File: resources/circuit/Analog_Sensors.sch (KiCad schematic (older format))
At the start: 43 parts, among them J3 Screw_Terminal_1x08, Q10 BSS138, Q11 BSS138, Q7 BSS138, Q8 BSS138, Q9 BSS138, U13 Airspeed, U14 Static Pressure, U15 MAP Pressure, U8 MCP3008, U9 MCP3008

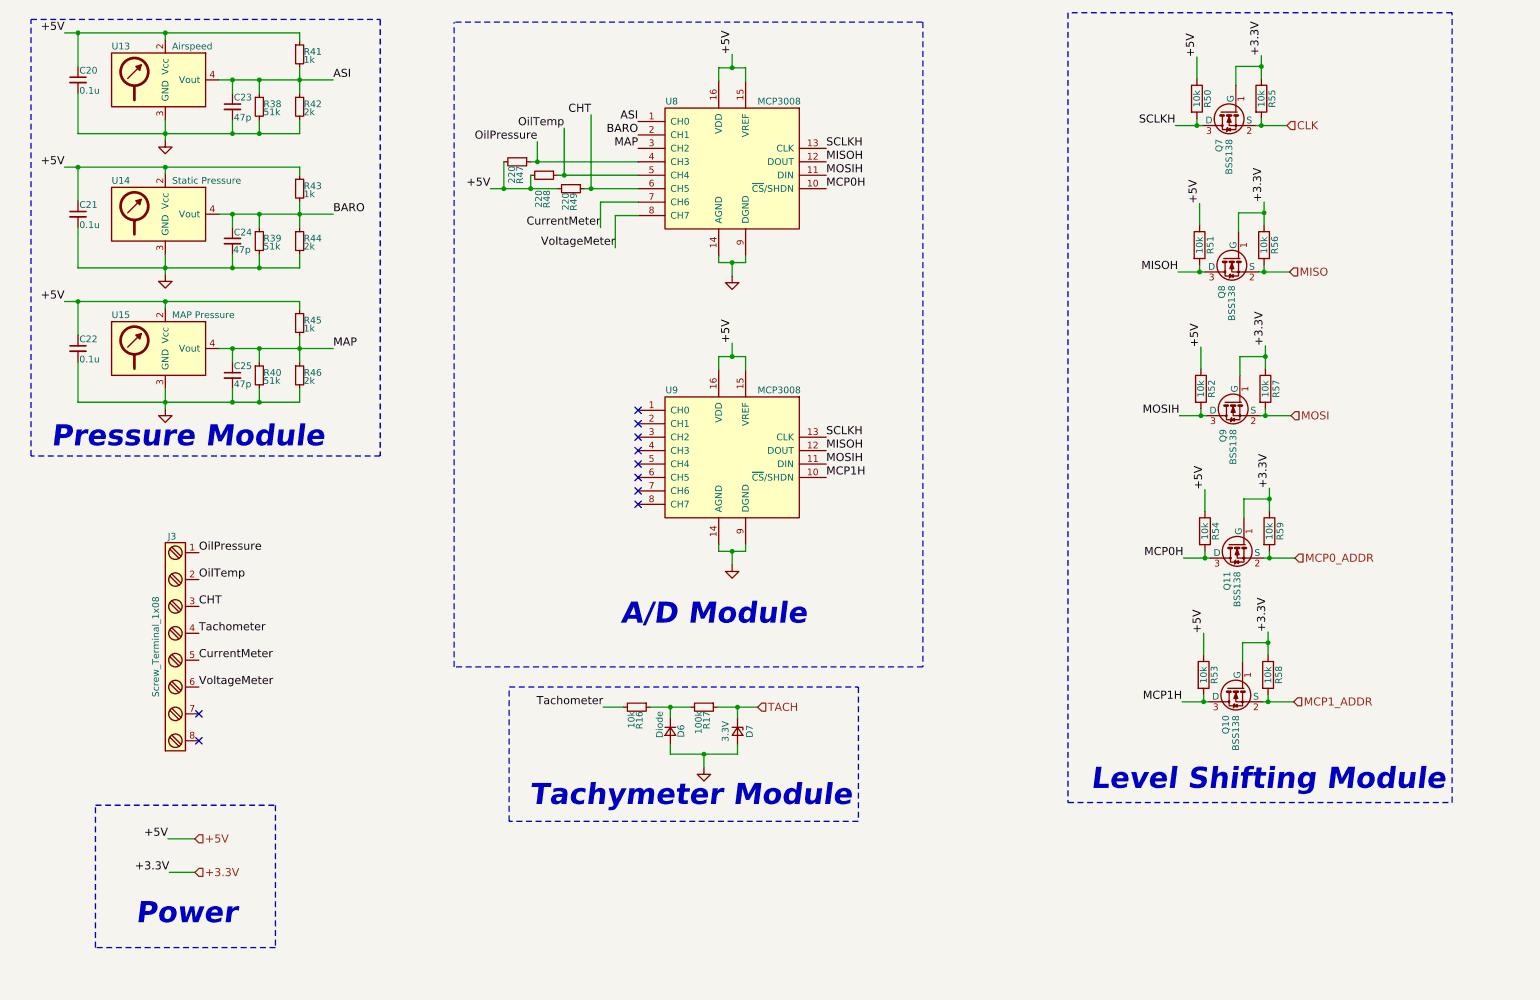
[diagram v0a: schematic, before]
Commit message: Another RPM reading solution
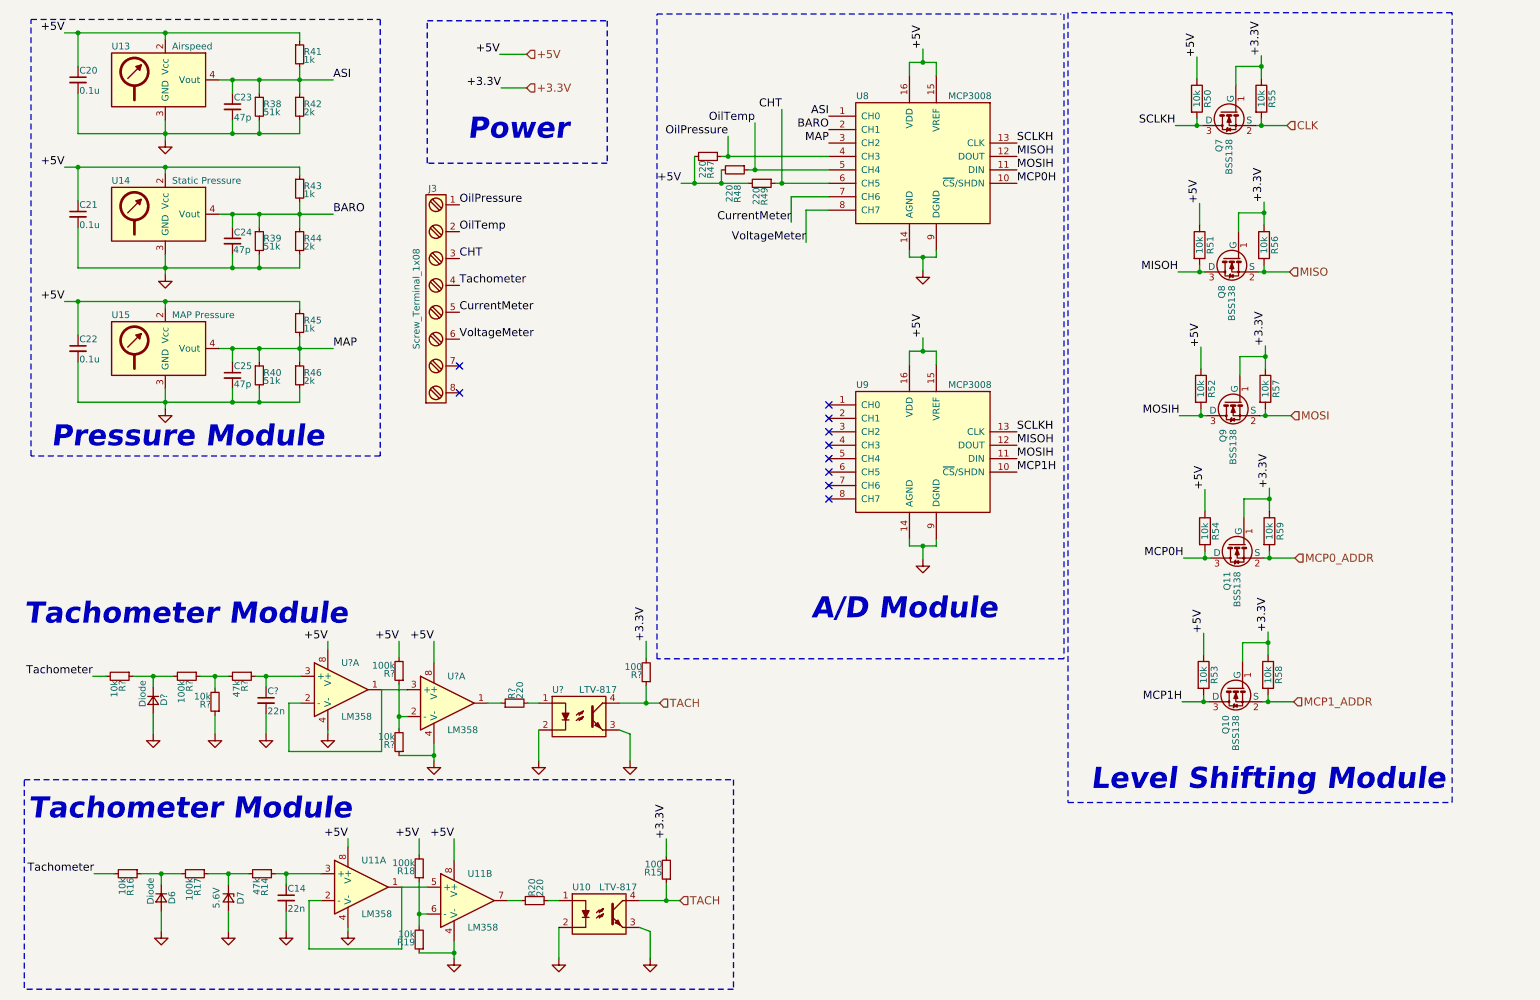
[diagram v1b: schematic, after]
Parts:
- added C14, C?: 22n, symbol C_Small
- added D?: Diode, Diodes_SMD:D_0603, symbol D_Small
- added R14, R?: 47k, symbol R_Small
- added R15, R?: 100, symbol R_Small
- added R18, R? (x2): 100k, Resistors_SMD:R_0603, symbol R_Small
- added R19, R? (x3): 10k, Resistors_SMD:R_0603, symbol R_Small
- added R20, R?: 220, Resistors_SMD:R_0603, symbol R_Small
- added U10, U?: LTV-817, Housings_DIP:DIP-4_W7.62mm, symbol LTV-817
- added U11, U? (x2): LM358, symbol LM358
- D7: value 3.3V -> 5.6V
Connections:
- net +3.3V: now also R15.2, R?.2
- net +5V: now also R18.2, R?.2, U11.8 (V+), U11.8 (V+), U?.8 (V+), U?.8 (V+)
- net GND: now also C14.2, C?.2, D?.2 (A), R19.1, R?.1, R?.1, U10.2, U10.3, U11.4 (V-), U11.4 (V-), U?.2, U?.3, U?.4 (V-), U?.4 (V-)
- net TACH: now also R15.1, R?.1, U10.4, U?.4; no longer D7.1 (K), R17.1
- net Tachometer: now also R?.2
- new net: D7.1 (K), R14.2, R17.1
- new net: C14.1, R14.1, U11.3 (+)
- new net: R20.2, U10.1
- new net: U11.1, U11.2 (-), U11.5 (+)
- new net: R18.1, R19.2, U11.6 (-)
- new net: R20.1, U11.7
- new net: R?.2, U?.1
- new net: U?.1, U?.2 (-), U?.3 (+)
- new net: C?.1, R?.1, U?.3 (+)
- new net: R?.1, U?.1
- new net: R?.1, R?.2, U?.2 (-)
- new net: D?.1 (K), R?.1, R?.2
- new net: R?.1, R?.2, R?.2
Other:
- note added: "Tachometer Module"
- note removed: "Tachymeter Module"
- moved on the sheet: D6, D7, J3, R16, R17, R47, R48, R49, U8, U9
